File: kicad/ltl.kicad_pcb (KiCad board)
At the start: 2 copper layers, 89.5 x 63.1 mm, 21 parts, among them J1 CONN_01X03, J2 BARREL_JACK, U1 ESP-12E, U2 DS18B20

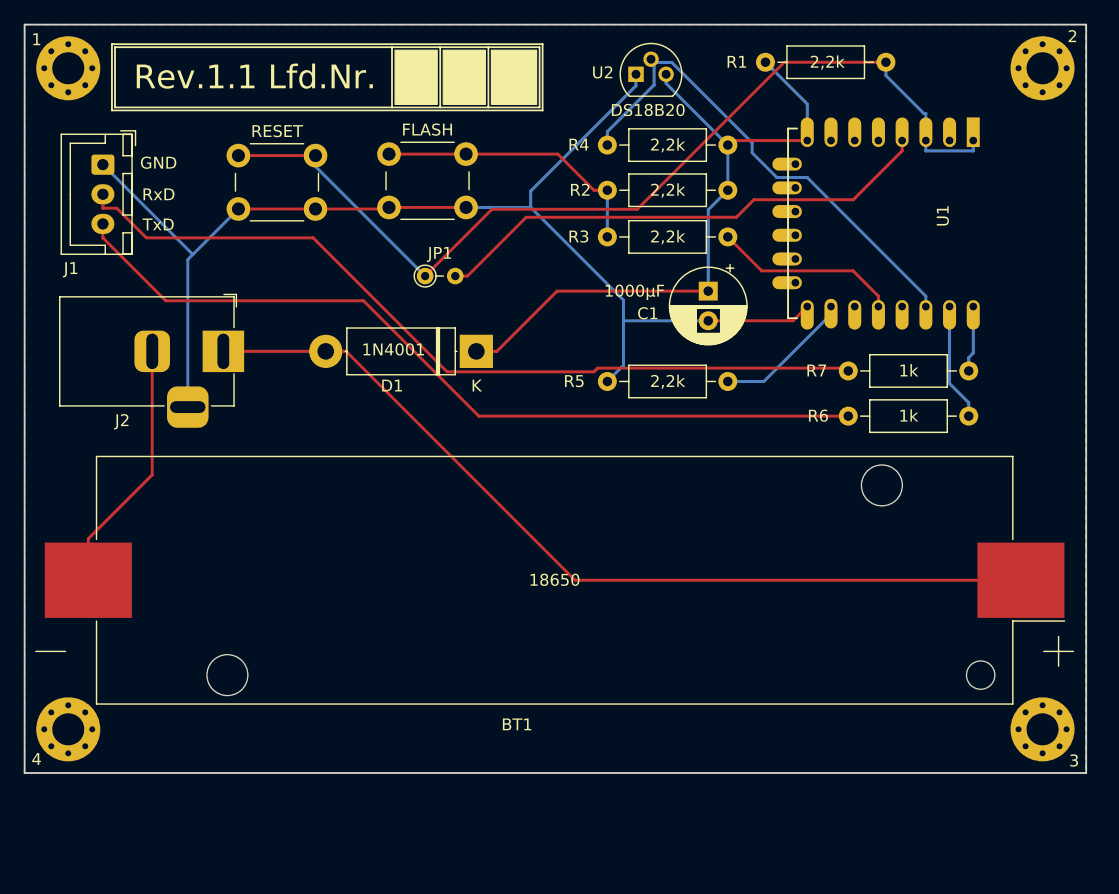
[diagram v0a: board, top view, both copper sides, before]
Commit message: Viele Änderungen, siehe Wiki
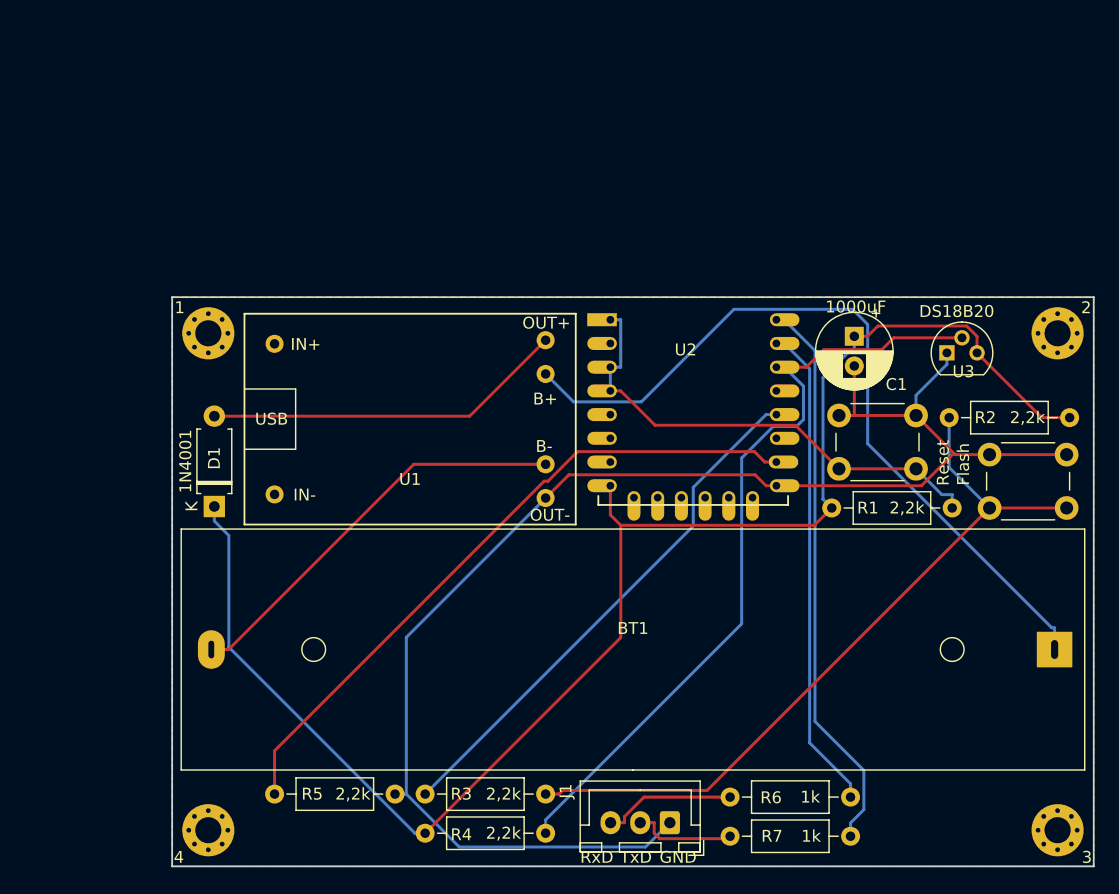
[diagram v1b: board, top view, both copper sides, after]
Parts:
- removed 1: 1, MountingHole:MountingHole_2.7mm_M2.5_Pad_Via
- removed 2: 2, MountingHole:MountingHole_2.7mm_M2.5_Pad_Via
- removed 3: 3, MountingHole:MountingHole_2.7mm_M2.5_Pad_Via
- removed 4: 4, MountingHole:MountingHole_2.7mm_M2.5_Pad_Via
- removed FLASH: SW_DIP_x02_LTL, Button_Switch_THT:SW_PUSH_6mm
- removed J2: BARREL_JACK, Connector_BarrelJack:BarrelJack_Horizontal
- removed JP1: Jumper, Resistor_THT:R_Axial_DIN0204_L3.6mm_D1.6mm_P2.54mm_Vertical
- added Flash: Flash, Button_Switch_THT:SW_PUSH_6mm, F.Cu at (161.5, 108.7)
- added MH_1: 1, MountingHole:MountingHole_2.2mm_M2_Pad_Via, F.Cu at (89.2, 94.0)
- added MH_2: 2, MountingHole:MountingHole_2.2mm_M2_Pad_Via, F.Cu at (160.8, 94.0)
- added MH_3: 3, MountingHole:MountingHole_2.2mm_M2_Pad_Via, F.Cu at (160.8, 135.9)
- added MH_4: 4, MountingHole:MountingHole_2.2mm_M2_Pad_Via, F.Cu at (89.2, 135.9)
- added U1: TP4056, TP4506:TP4056, F.Cu at (106.2, 101.2)
- BT1: footprint Battery:BatteryHolder_Keystone_1042_1x18650 -> 18650:18650_small
- C1: value 1000µF -> 1000uF
- D1: footprint Diode_THT:D_5W_P12.70mm_Horizontal -> Diode_THT:D_A-405_P7.62mm_Horizontal
- Reset: renamed from RESET; value SW_DIP_x02_LTL -> Reset
- moved J1 73.3 mm to (128.1, 135.3), turned to 180 degrees
- moved R4 63.4 mm to (107.4, 136.1), turned to 0 degrees
- moved Reset 63.0 mm to (148.8, 105.4), turned to 180 degrees
- moved R3 53.5 mm to (107.4, 132.8), turned to 0 degrees
- moved R7 40.5 mm to (133.2, 136.4)
- moved R5 39.1 mm to (104.9, 132.8), turned to 180 degrees
- moved R1 38.0 mm to (141.7, 108.7)
- moved U3 35.2 mm to (151.4, 95.6)
- moved R2 34.6 mm to (161.8, 101.1)
- moved U2 34.1 mm to (123.1, 92.8), turned to 0 degrees
- moved R6 33.6 mm to (133.2, 133.1)
- moved D1 25.7 mm to (89.7, 108.6), turned to 90 degrees
- moved C1 12.9 mm to (143.6, 94.2)
- moved BT1 8.82 mm to (125.0, 120.7)
- renumbered U1 to U2, U2 to U3
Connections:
- D1 pad 2: Net-(BT1-Pad1) -> Net-(D1-Pad2)
- R1 pad 2: Net-(JP1-Pad1) -> Net-(R1-Pad2)
- Reset pad 1: Net-(JP1-Pad1) -> Net-(R1-Pad2)
- U2 pad 1: Net-(JP1-Pad1) -> Net-(R1-Pad2)
- U2 pad 3: Net-(JP1-Pad1) -> Net-(R1-Pad2)
- U2 pad 4: Net-(JP1-Pad2) -> Net-(R1-Pad2)
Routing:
- net Net-(JP1-Pad1): track 80.7 -> 0.00 mm
- net +3V3: track 57.7 -> 128.9 mm
- net /TxD: track 70.0 -> 8.74 mm
- net /RxD: track 70.3 -> 11.3 mm
- net Net-(R5-Pad2): track 11.7 -> 56.8 mm
- net Net-(JP1-Pad2): track 42.9 -> 0.00 mm
- net Net-(R7-Pad2): track 5.59 -> 47.5 mm
- net Net-(R1-Pad2): track 0.00 -> 41.3 mm
- net Net-(Flash1-Pad1): track 23.6 -> 63.0 mm
- net Net-(R6-Pad2): track 9.91 -> 41.2 mm
- net Net-(D1-Pad2): track 0.00 -> 30.6 mm
- net Net-(R3-Pad1): track 15.6 -> 44.8 mm
- net Net-(R4-Pad2): track 41.4 -> 67.5 mm
- net GND: track 103.3 -> 123.6 mm
- net Net-(BT1-Pad2): track 21.5 -> 34.7 mm
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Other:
- board size 89.5 x 63.1 mm -> 77.7 x 48 mm
- board text added: "Rev.1.2 Lfd.Nr."
- board text removed: "Rev.1.1 Lfd.Nr."

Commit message: ch ch ch changes
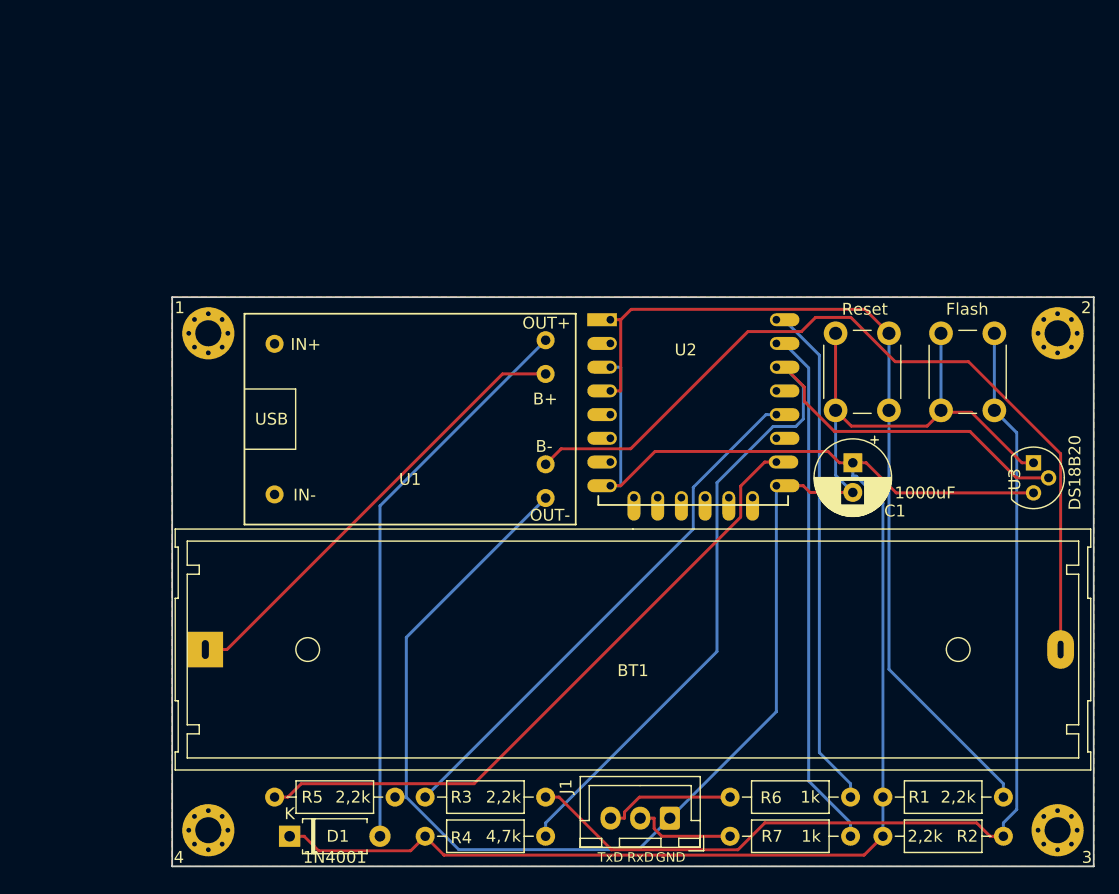
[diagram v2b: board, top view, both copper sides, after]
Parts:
- R4: value 2,2k -> 4,7k
- moved R2 38.7 mm to (146.1, 136.4), turned to 0 degrees
- moved D1 28.5 mm to (96.0, 136.4), turned to 0 degrees
- moved R1 24.8 mm to (146.1, 133.1)
- moved Flash 15.9 mm to (155.4, 94.0), turned to 270 degrees
- moved U3 11.8 mm to (158.8, 104.9), turned to 270 degrees
- moved Reset 11.7 mm to (146.6, 94.0), turned to 270 degrees
- moved C1 10.7 mm to (143.5, 104.9)
- moved J1 0.38 mm to (128.1, 134.9)
- moved R3 0.25 mm to (107.4, 133.1)
- moved R4 0.25 mm to (107.4, 136.4)
- moved R5 0.25 mm to (104.9, 133.1)
- turned BT1 to 0 degrees
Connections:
- J1 pad 2: /TxD -> /RxD
- J1 pad 3: /RxD -> /TxD
- R6 pad 1: /RxD -> /TxD
- R7 pad 1: /TxD -> /RxD
- U2 pad 15: Net-(R6-Pad2) -> Net-(R7-Pad2)
- U2 pad 16: Net-(R7-Pad2) -> Net-(R6-Pad2)
- U2 pad 3: Net-(R1-Pad2) -> +3V3
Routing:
- net Net-(BT1-Pad2): track 34.7 -> 69.8 mm
- net Net-(R1-Pad2): track 41.3 -> 74.7 mm
- net Net-(BT1-Pad1): track 66.0 -> 38.3 mm
- net Net-(Flash1-Pad1): track 63.0 -> 85.5 mm
- net Net-(D1-Pad2): track 30.6 -> 47.6 mm
- net GND: track 123.6 -> 134.8 mm
- net Net-(R4-Pad2): track 67.5 -> 78.5 mm
- net +3V3: track 128.9 -> 135.2 mm
- net Net-(R7-Pad2): track 47.5 -> 44.5 mm
- net /RxD: track 11.3 -> 8.73 mm
- net /TxD: track 8.74 -> 11.1 mm
- net Net-(R6-Pad2): track 41.2 -> 43.2 mm
- net Net-(R5-Pad2): track 56.8 -> 55.6 mm
- added copper zone on B.Cu, net (none)
- removed copper zone on B.Cu, net GND
